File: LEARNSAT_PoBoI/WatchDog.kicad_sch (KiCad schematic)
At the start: 12 parts, among them SW1 B3U-1000P, SW2 B3U-1000P, U1 MAX6746KA29+T, U2 SN74AUP1G08QDCKRQ1, U3 MAX6746KA29+T, U4 SN74AUP1G08QDCKRQ1

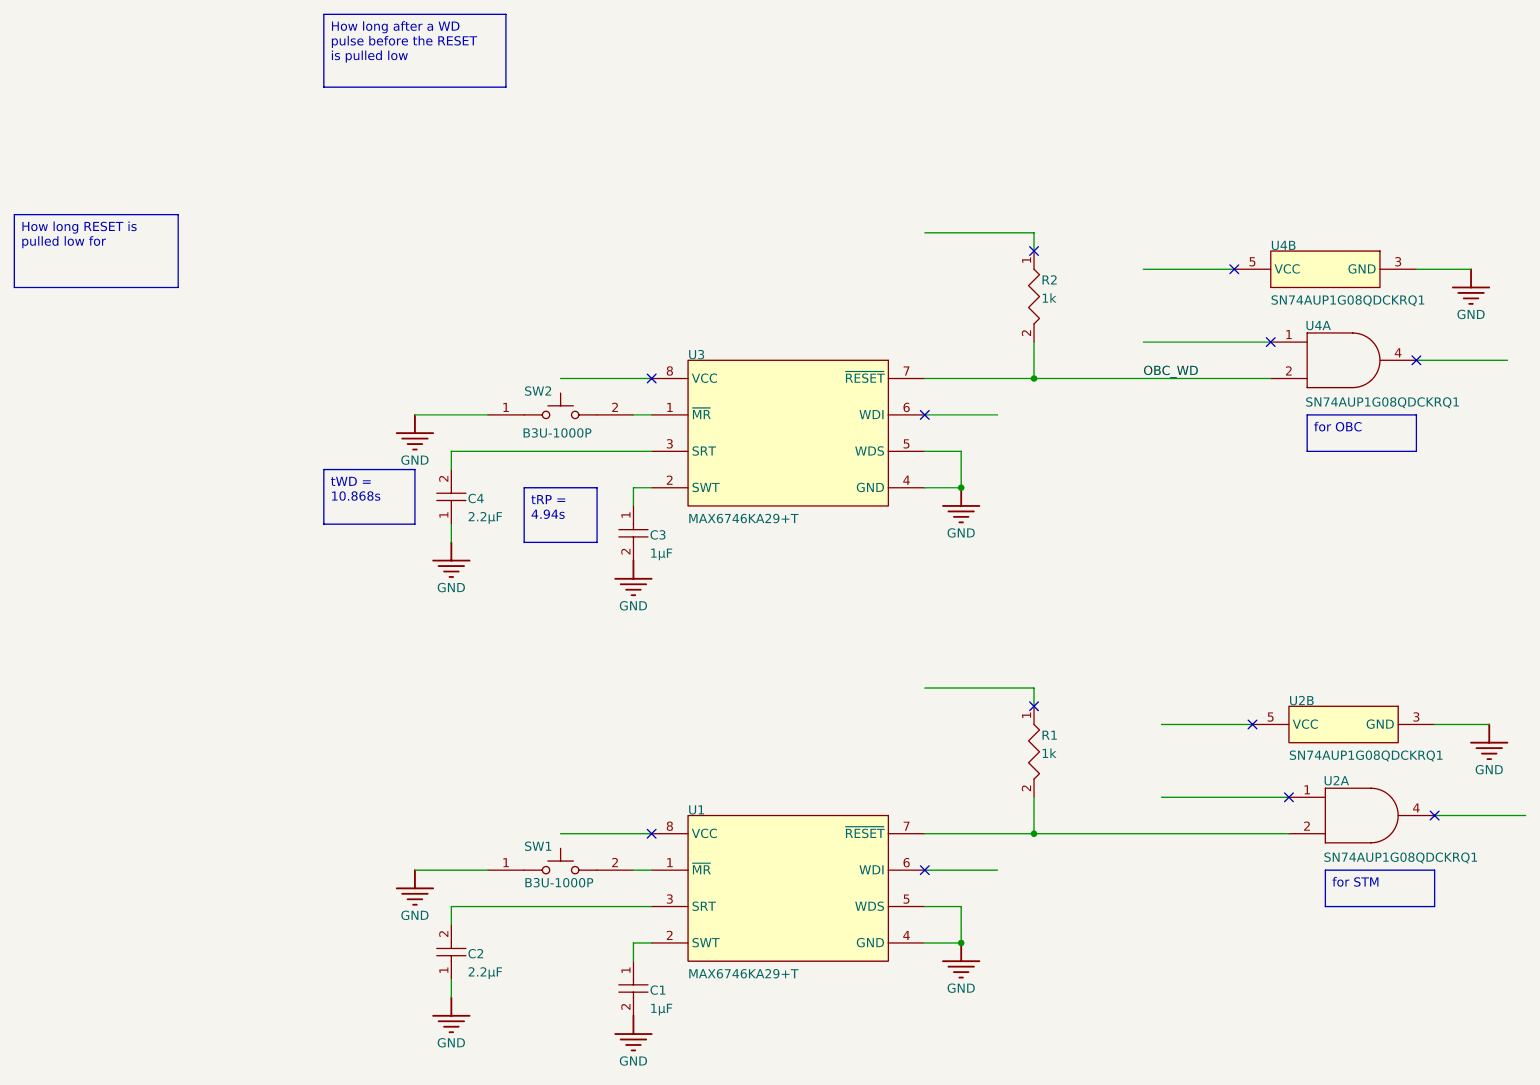
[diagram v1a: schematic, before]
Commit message: Added footprints
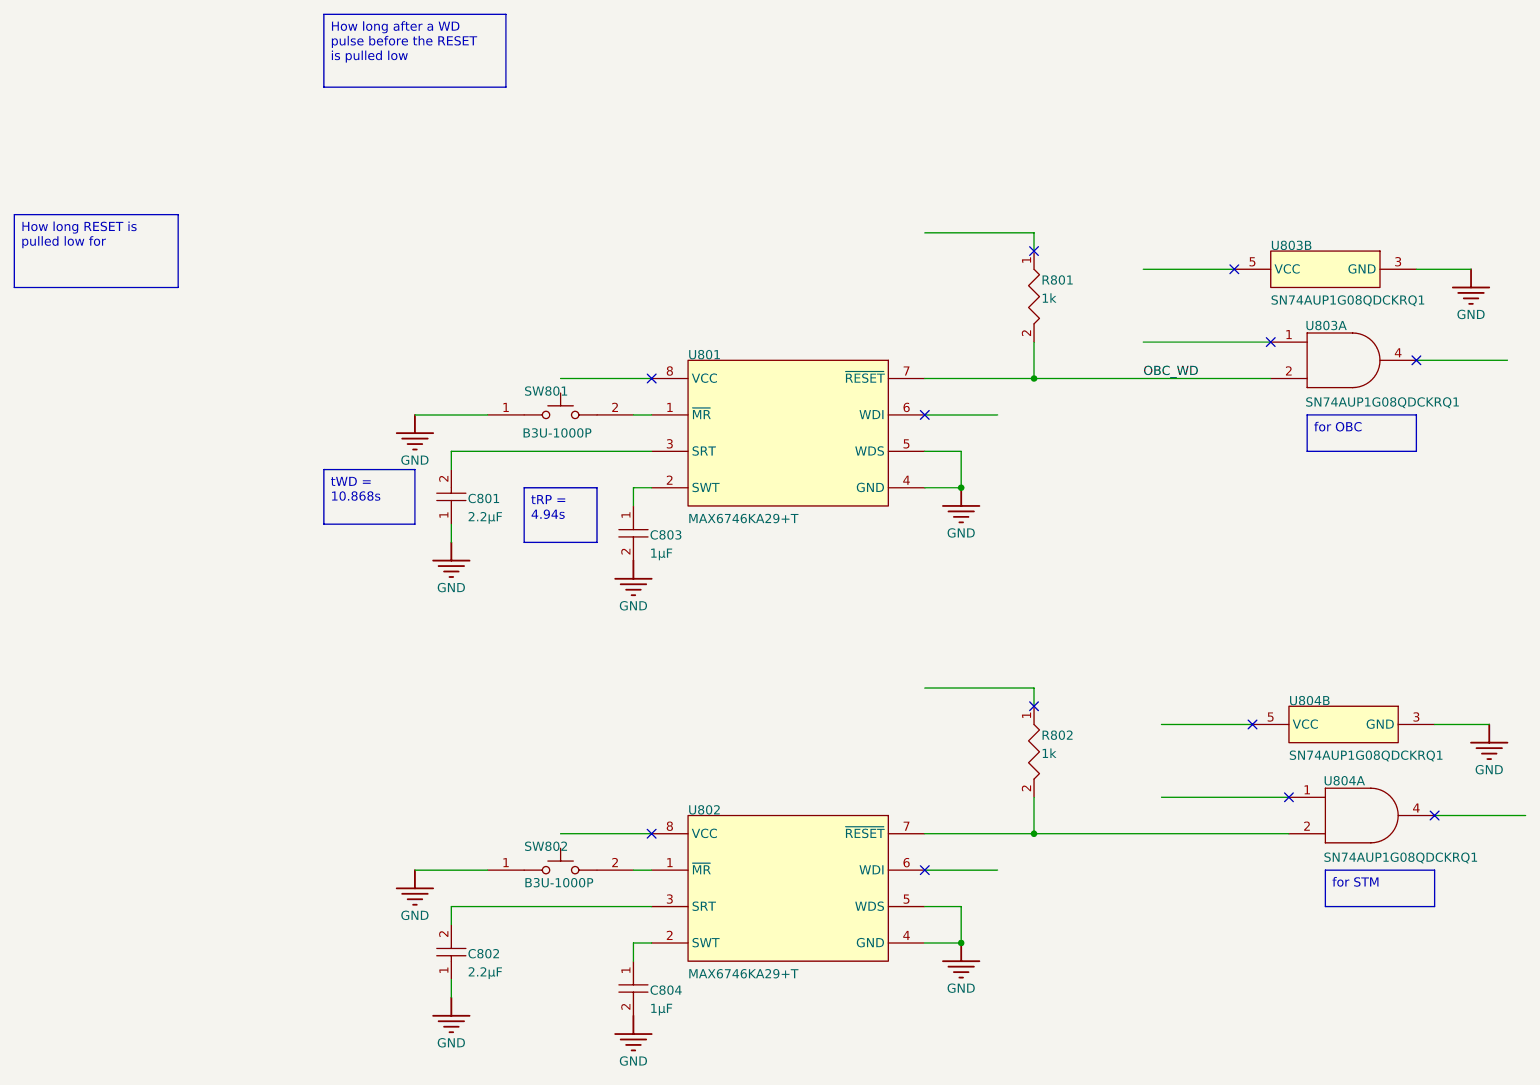
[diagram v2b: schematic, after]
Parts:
- C801: renamed from C4; footprint CAPC0402(1005)60_L -> Capacitor_SMD:C_0402_1005Metric
- C802: renamed from C2; footprint CAPC0402(1005)60_L -> Capacitor_SMD:C_0402_1005Metric
- C803: renamed from C3; footprint CAPC0603(1608)100_L -> Capacitor_SMD:C_0603_1608Metric
- C804: renamed from C1; footprint CAPC0603(1608)100_L -> Capacitor_SMD:C_0603_1608Metric
- R801: renamed from R2; footprint RESC0805(2012)_L -> Resistor_SMD:R_0805_2012Metric
- R802: renamed from R1; footprint RESC0805(2012)_L -> Resistor_SMD:R_0805_2012Metric
- SW801: renamed from SW2; footprint OMRON-B3U-1000_V -> B3U-1000P:SW_B3U-1000P
- SW802: renamed from SW1; footprint OMRON-B3U-1000_V -> B3U-1000P:SW_B3U-1000P
- U801: renamed from U3; footprint FP-K8-5-IPC_C -> MAX6746KA29_T:SOT65P280X145-8N
- U802: renamed from U1; footprint FP-K8-5-IPC_C -> MAX6746KA29_T:SOT65P280X145-8N
- U803: renamed from U4; footprint DCK0005A_N -> SN74AUP1G08QDCKRQ1:SOT65P210X110-5N
- U804: renamed from U2; footprint DCK0005A_N -> SN74AUP1G08QDCKRQ1:SOT65P210X110-5N
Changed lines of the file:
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@@
 		(on_board yes)
 		(dnp no)
-		(property "Reference" "#PWR?"
+		(property "Reference" "#PWR0806"
 			(at 96.52 172.72 0)
 			(effects
@@
 			(project ""
 				(path "/31302da5-a970-4b2b-aa05-afcd06cb9d09/24205a11-7394-4676-a8e1-3f02d7a9d0eb"
-					(reference "#PWR?")
+					(reference "#PWR0806")
 					(unit 1)
 				)
@@
 		(on_board yes)
 		(dnp no)
-		(property "Reference" "R1"
+		(property "Reference" "R802"
 			(at 153.416 134.366 0)
 			(effects
@@
 			)
 		)
-		(property "Footprint" "RESC0805(2012)_L"
+		(property "Footprint" "Resistor_SMD:R_0805_2012Metric"
 			(at 152.4 129.54 0)
 			(effects
@@
 			(project ""
 				(path "/31302da5-a970-4b2b-aa05-afcd06cb9d09/24205a11-7394-4676-a8e1-3f02d7a9d0eb"
-					(reference "R1")
+					(reference "R802")
 					(unit 1)
 				)
@@
 		(on_board yes)
 		(dnp no)
-		(property "Reference" "C3"
+		(property "Reference" "C803"
 			(at 98.806 106.426 0)
 			(effects
@@
 			)
 		)
-		(property "Footprint" "CAPC0603(1608)100_L"
+		(property "Footprint" "Capacitor_SMD:C_0603_1608Metric"
 			(at 96.52 101.6 0)
 			(effects
@@
 			(project ""
 				(path "/31302da5-a970-4b2b-aa05-afcd06cb9d09/24205a11-7394-4676-a8e1-3f02d7a9d0eb"
-					(reference "C3")
+					(reference "C803")
 					(unit 1)
 				)
@@
 		(on_board yes)
 		(dnp no)
-		(property "Reference" "#PWR?"
+		(property "Reference" "#PWR0807"
 			(at 142.24 99.06 0)
 			(effects
@@
 			(project ""
 				(path "/31302da5-a970-4b2b-aa05-afcd06cb9d09/24205a11-7394-4676-a8e1-3f02d7a9d0eb"
-					(reference "#PWR?")
+					(reference "#PWR0807")
 					(unit 1)
 				)
@@
 		(on_board yes)
 		(dnp no)
-		(property "Reference" "C1"
+		(property "Reference" "C804"
 			(at 98.806 169.926 0)
 			(effects
@@
 			)
 		)
-		(property "Footprint" "CAPC0603(1608)100_L"
+		(property "Footprint" "Capacitor_SMD:C_0603_1608Metric"
 			(at 96.52 165.1 0)
 			(effects
@@
 			(project ""
 				(path "/31302da5-a970-4b2b-aa05-afcd06cb9d09/24205a11-7394-4676-a8e1-3f02d7a9d0eb"
-					(reference "C1")
+					(reference "C804")
 					(unit 1)
 				)
@@
 		(on_board yes)
 		(dnp no)
-		(property "Reference" "R2"
+		(property "Reference" "R801"
 			(at 153.416 70.866 0)
 			(effects
@@
 			)
 		)
-		(property "Footprint" "RESC0805(2012)_L"
+		(property "Footprint" "Resistor_SMD:R_0805_2012Metric"
 			(at 152.4 66.04 0)
 			(effects
@@
 			(project ""
 				(path "/31302da5-a970-4b2b-aa05-afcd06cb9d09/24205a11-7394-4676-a8e1-3f02d7a9d0eb"
-					(reference "R2")
+					(reference "R801")
 					(unit 1)
 				)
@@
 		(on_board yes)
 		(dnp no)
-		(property "Reference" "C2"
+		(property "Reference" "C802"
 			(at 73.406 164.846 0)
 			(effects
@@
 			)
 		)
-		(property "Footprint" "CAPC0402(1005)60_L"
+		(property "Footprint" "Capacitor_SMD:C_0402_1005Metric"
 			(at 71.12 167.64 0)
 			(effects
@@
 			(project ""
 				(path "/31302da5-a970-4b2b-aa05-afcd06cb9d09/24205a11-7394-4676-a8e1-3f02d7a9d0eb"
-					(reference "C2")
+					(reference "C802")
 					(unit 1)
 				)
@@
 		(on_board yes)
 		(dnp no)
-		(property "Reference" "#PWR?"
+		(property "Reference" "#PWR0804"
 			(at 71.12 170.18 0)
 			(effects
@@
 			(project ""
 				(path "/31302da5-a970-4b2b-aa05-afcd06cb9d09/24205a11-7394-4676-a8e1-3f02d7a9d0eb"
-					(reference "#PWR?")
+					(reference "#PWR0804")
 					(unit 1)
 				)
@@
 		(on_board yes)
 		(dnp no)
-		(property "Reference" "#PWR?"
+		(property "Reference" "#PWR0802"
 			(at 66.04 152.4 0)
 			(effects
@@
 			(project ""
 				(path "/31302da5-a970-4b2b-aa05-afcd06cb9d09/24205a11-7394-4676-a8e1-3f02d7a9d0eb"
-					(reference "#PWR?")
+					(reference "#PWR0802")
 					(unit 1)
 				)
@@
 		(on_board yes)
 		(dnp no)
-		(property "Reference" "U3"
+		(property "Reference" "U801"
 			(at 104.14 81.28 0)
 			(effects
@@
 			)
 		)
-		(property "Footprint" "FP-K8-5-IPC_C"
+		(property "Footprint" "MAX6746KA29_T:SOT65P280X145-8N"
 			(at 99.06 83.82 0)
 			(effects
@@
 			(project ""
 				(path "/31302da5-a970-4b2b-aa05-afcd06cb9d09/24205a11-7394-4676-a8e1-3f02d7a9d0eb"
-					(reference "U3")
+					(reference "U801")
 					(unit 1)
 				)
@@
 		(on_board yes)
 		(dnp no)
-		(property "Reference" "#PWR?"
+		(property "Reference" "#PWR0803"
 			(at 71.12 106.68 0)
 			(effects
@@
 			(project ""
 				(path "/31302da5-a970-4b2b-aa05-afcd06cb9d09/24205a11-7394-4676-a8e1-3f02d7a9d0eb"
-					(reference "#PWR?")
+					(reference "#PWR0803")
 					(unit 1)
 				)
@@
 		(on_board yes)
 		(dnp no)
-		(property "Reference" "U4"
+		(property "Reference" "U803"
 			(at 185.42 66.04 0)
 			(effects
@@
 			)
 		)
-		(property "Footprint" "DCK0005A_N"
+		(property "Footprint" "SN74AUP1G08QDCKRQ1:SOT65P210X110-5N"
 			(at 185.42 66.04 0)
 			(effects
@@
 			(project ""
 				(path "/31302da5-a970-4b2b-aa05-afcd06cb9d09/24205a11-7394-4676-a8e1-3f02d7a9d0eb"
-					(reference "U4")
+					(reference "U803")
 					(unit 2)
 				)
@@
 		(on_board yes)
 		(dnp no)
-		(property "Reference" "C4"
+		(property "Reference" "C801"
 			(at 73.406 101.346 0)
 			(effects
@@
 			)
 		)
-		(property "Footprint" "CAPC0402(1005)60_L"
+		(property "Footprint" "Capacitor_SMD:C_0402_1005Metric"
 			(at 71.12 104.14 0)
 			(effects
@@
 			(project ""
 				(path "/31302da5-a970-4b2b-aa05-afcd06cb9d09/24205a11-7394-4676-a8e1-3f02d7a9d0eb"
-					(reference "C4")
+					(reference "C801")
 					(unit 1)
 				)
@@
 		(on_board yes)
 		(dnp no)
-		(property "Reference" "#PWR?"
+		(property "Reference" "#PWR0810"
 			(at 215.9 132.08 0)
 			(effects
@@
 			(project ""
 				(path "/31302da5-a970-4b2b-aa05-afcd06cb9d09/24205a11-7394-4676-a8e1-3f02d7a9d0eb"
-					(reference "#PWR?")
+					(reference "#PWR0810")
 					(unit 1)
 				)
@@
 		(on_board yes)
 		(dnp no)
-		(property "Reference" "SW2"
+		(property "Reference" "SW801"
 			(at 81.28 86.36 0)
 			(effects
@@
 			)
 		)
-		(property "Footprint" "OMRON-B3U-1000_V"
+		(property "Footprint" "B3U-1000P:SW_B3U-1000P"
 			(at 81.28 86.36 0)
 			(effects
@@
 			(project ""
 				(path "/31302da5-a970-4b2b-aa05-afcd06cb9d09/24205a11-7394-4676-a8e1-3f02d7a9d0eb"
-					(reference "SW2")
+					(reference "SW801")
 					(unit 1)
 				)
@@
 		(on_board yes)
 		(dnp no)
-		(property "Reference" "#PWR?"
+		(property "Reference" "#PWR0808"
 			(at 142.24 162.56 0)
 			(effects
@@
 			(project ""
 				(path "/31302da5-a970-4b2b-aa05-afcd06cb9d09/24205a11-7394-4676-a8e1-3f02d7a9d0eb"
-					(reference "#PWR?")
+					(reference "#PWR0808")
 					(unit 1)
 				)
@@
 		(on_board yes)
 		(dnp no)
-		(property "Reference" "#PWR?"
+		(property "Reference" "#PWR0805"
 			(at 96.52 109.22 0)
 			(effects
@@
 			(project ""
 				(path "/31302da5-a970-4b2b-aa05-afcd06cb9d09/24205a11-7394-4676-a8e1-3f02d7a9d0eb"
-					(reference "#PWR?")
+					(reference "#PWR0805")
 					(unit 1)
 				)
@@
 		(on_board yes)
 		(dnp no)
-		(property "Reference" "#PWR?"
+		(property "Reference" "#PWR0809"
 			(at 213.36 68.58 0)
 			(effects
@@
 			(project ""
 				(path "/31302da5-a970-4b2b-aa05-afcd06cb9d09/24205a11-7394-4676-a8e1-3f02d7a9d0eb"
-					(reference "#PWR?")
+					(reference "#PWR0809")
 					(unit 1)
 				)
@@
 		(on_board yes)
 		(dnp no)
-		(property "Reference" "U2"
+		(property "Reference" "U804"
 			(at 192.786 140.716 0)
 			(effects
@@
 			)
 		)
-		(property "Footprint" "DCK0005A_N"
+		(property "Footprint" "SN74AUP1G08QDCKRQ1:SOT65P210X110-5N"
 			(at 193.04 139.7 0)
 			(effects
@@
 			(project ""
 				(path "/31302da5-a970-4b2b-aa05-afcd06cb9d09/24205a11-7394-4676-a8e1-3f02d7a9d0eb"
-					(reference "U2")
+					(reference "U804")
 					(unit 1)
 				)
@@
 		(on_board yes)
 		(dnp no)
-		(property "Reference" "#PWR?"
+		(property "Reference" "#PWR0801"
 			(at 66.04 88.9 0)
 			(effects
@@
 			(project ""
 				(path "/31302da5-a970-4b2b-aa05-afcd06cb9d09/24205a11-7394-4676-a8e1-3f02d7a9d0eb"
-					(reference "#PWR?")
+					(reference "#PWR0801")
 					(unit 1)
 				)
@@
 		(on_board yes)
 		(dnp no)
-		(property "Reference" "U4"
+		(property "Reference" "U803"
 			(at 190.246 77.216 0)
 			(effects
@@
 			)
 		)
-		(property "Footprint" "DCK0005A_N"
+		(property "Footprint" "SN74AUP1G08QDCKRQ1:SOT65P210X110-5N"
 			(at 190.5 76.2 0)
 			(effects
@@
 			(project ""
 				(path "/31302da5-a970-4b2b-aa05-afcd06cb9d09/24205a11-7394-4676-a8e1-3f02d7a9d0eb"
-					(reference "U4")
+					(reference "U803")
 					(unit 1)
 				)
@@
 		(on_board yes)
 		(dnp no)
-		(property "Reference" "U2"
+		(property "Reference" "U804"
 			(at 187.96 129.54 0)
 			(effects
@@
 			)
 		)
-		(property "Footprint" "DCK0005A_N"
+		(property "Footprint" "SN74AUP1G08QDCKRQ1:SOT65P210X110-5N"
 			(at 187.96 129.54 0)
 			(effects
@@
 			(project ""
 				(path "/31302da5-a970-4b2b-aa05-afcd06cb9d09/24205a11-7394-4676-a8e1-3f02d7a9d0eb"
-					(reference "U2")
+					(reference "U804")
 					(unit 2)
 				)
@@
 		(on_board yes)
 		(dnp no)
-		(property "Reference" "SW1"
+		(property "Reference" "SW802"
 			(at 81.28 149.86 0)
 			(effects
@@
 			)
 		)
-		(property "Footprint" "OMRON-B3U-1000_V"
+		(property "Footprint" "B3U-1000P:SW_B3U-1000P"
 			(at 81.28 149.86 0)
 			(effects
@@
 			(project ""
 				(path "/31302da5-a970-4b2b-aa05-afcd06cb9d09/24205a11-7394-4676-a8e1-3f02d7a9d0eb"
-					(reference "SW1")
+					(reference "SW802")
 					(unit 1)
 				)
@@
 		(on_board yes)
 		(dnp no)
-		(property "Reference" "U1"
+		(property "Reference" "U802"
 			(at 104.14 144.78 0)
 			(effects
@@
 			)
 		)
-		(property "Footprint" "FP-K8-5-IPC_C"
+		(property "Footprint" "MAX6746KA29_T:SOT65P280X145-8N"
 			(at 99.06 147.32 0)
 			(effects
@@
 			(project ""
 				(path "/31302da5-a970-4b2b-aa05-afcd06cb9d09/24205a11-7394-4676-a8e1-3f02d7a9d0eb"
-					(reference "U1")
+					(reference "U802")
 					(unit 1)
 				)
